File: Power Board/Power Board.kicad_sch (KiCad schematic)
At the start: 126 parts, among them IC1 LTC4151IMS#PBF, J8 Conn_01x02, K1 Relay_DPST-NO, Q10 Q_NMOS_GDS, Q11 Q_NMOS_GDS, Q12 Q_NMOS_GDS, Q13 Q_NMOS_GDS, Q14 Q_NMOS_GDS, Q15 Q_NMOS_GDS, Q16 Q_NMOS_GDS, Q17 Q_NMOS_GDS, Q18 Q_NMOS_GDS, Q19 Q_NMOS_GDS, Q20 Q_NMOS_GDS, Q21 Q_NMOS_GDS, Q22 Q_NMOS_GDS, Q9 Q_NMOS_GDS, Q9 Q_PMOS_GDS, U1 ADR395, U10 LTC4372, U11 ACS770xCB-200U-PFF, U2 LTC4372, U3 LTC4372, U4 LTC4372, U5 LTC4372, U6 LTC4372, U7 LTC4372, U8 ADC128S052CIMT, U9 L7805

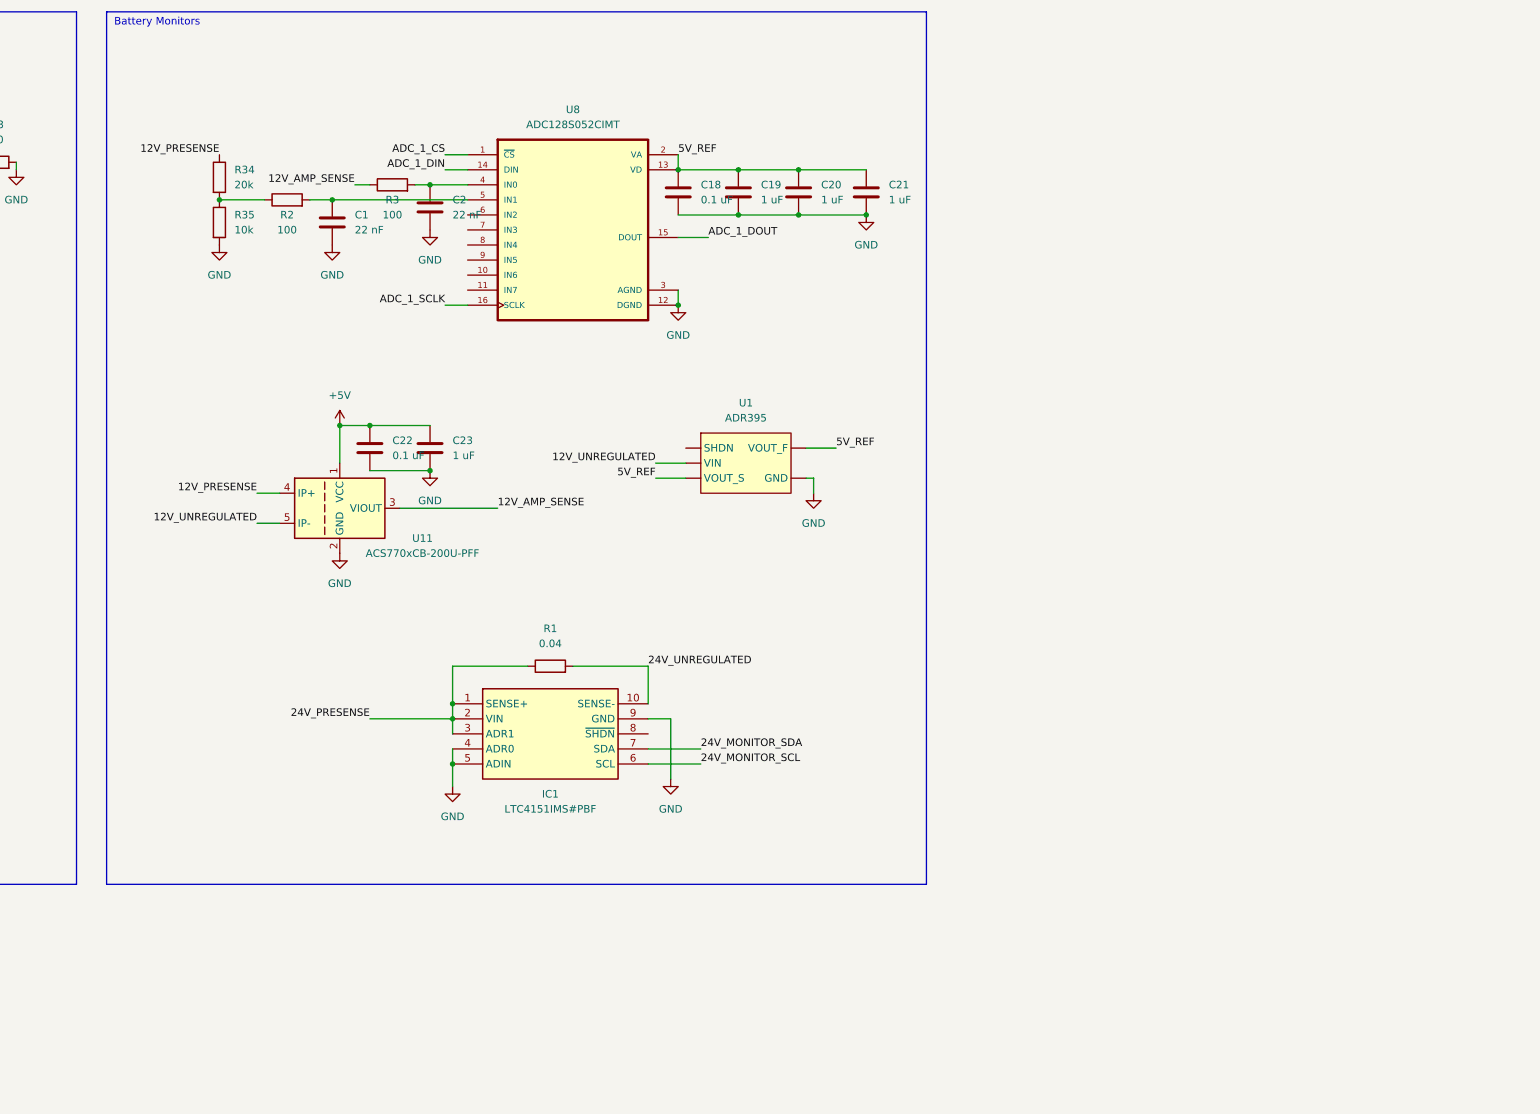
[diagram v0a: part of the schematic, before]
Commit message: working on power board
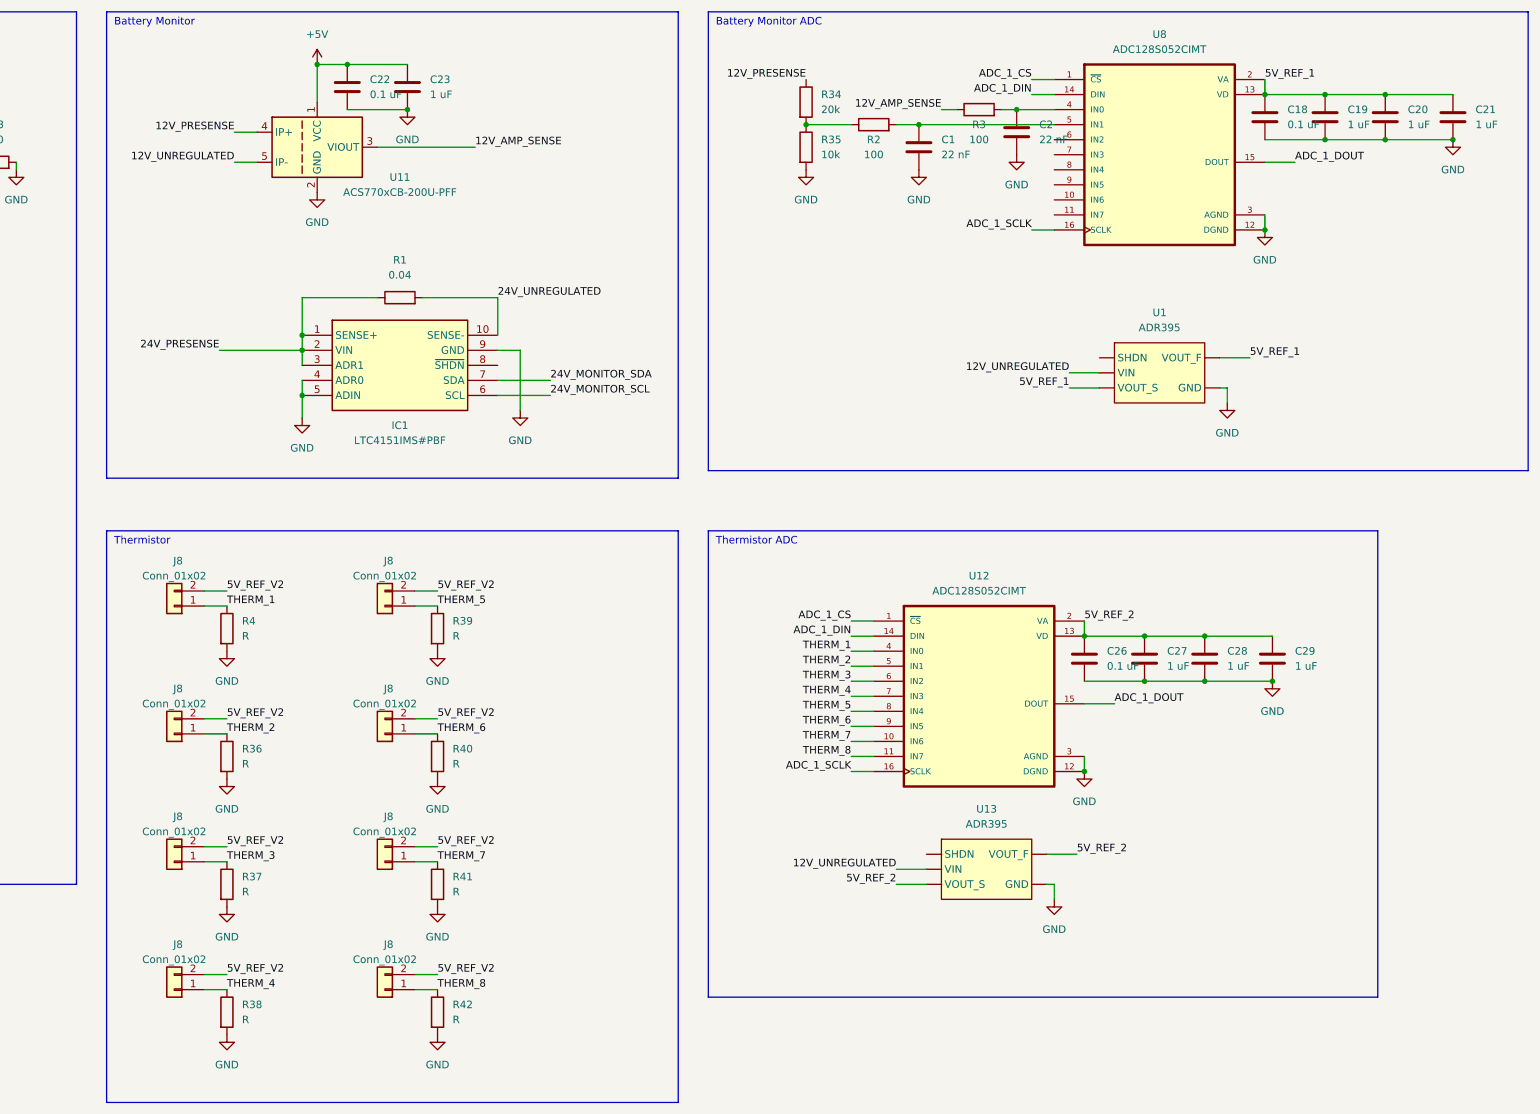
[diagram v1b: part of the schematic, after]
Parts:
- added C26: 0.1 uF, symbol Device:C
- added C27, C28, C29: 1 uF, symbol Device:C
- added J8 (x8): Conn_01x02, SOCMonitor:MOLEX_768290102, symbol Connector_Generic:Conn_01x02
- added R36, R37, R38, R39, R4, R40, R41, R42: R, symbol Device:R
- added U12: ADC128S052CIMT, ADC128S052CIMT:SOP65P640X120-16N, symbol ADC128S052CIMT:ADC128S052CIMT
- added U13: ADR395, Package_TO_SOT_SMD:SOT-23-5, symbol ADR395:ADR395
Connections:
- net 12V_UNREGULATED: now also U13. (VOUT_S)
- net ADC_1_CS: now also U12.1 (~{CS})
- net ADC_1_DIN: now also U12.14 (DIN)
- net ADC_1_DOUT: now also U12.15 (DOUT)
- net ADC_1_SCLK: now also U12.16 (SCLK)
- net GND: now also C26.2, C27.2, C28.2, C29.2, R36.2, R37.2, R38.2, R39.2, R4.2, R40.2, R41.2, R42.2, U12.12 (DGND), U12.3 (AGND), U13. (VOUT_S)
- net 5V_REF renamed 5V_REF_1
- new net 5V_REF_2: C26.1, C27.1, C28.1, C29.1, U12.13 (VD), U12.2 (VA), U13. (VOUT_S)
- new net 5V_REF_V2: J8.2 (Pin_2), J8.2 (Pin_2), J8.2 (Pin_2), J8.2 (Pin_2), J8.2 (Pin_2), J8.2 (Pin_2), J8.2 (Pin_2), J8.2 (Pin_2)
- new net THERM_1: J8.1 (Pin_1), R4.1, U12.4 (IN0)
- new net THERM_2: J8.1 (Pin_1), R36.1, U12.5 (IN1)
- new net THERM_3: J8.1 (Pin_1), R37.1, U12.6 (IN2)
- new net THERM_4: J8.1 (Pin_1), R38.1, U12.7 (IN3)
- new net THERM_5: J8.1 (Pin_1), R39.1, U12.8 (IN4)
- new net THERM_6: J8.1 (Pin_1), R40.1, U12.9 (IN5)
- new net THERM_7: J8.1 (Pin_1), R41.1, U12.10 (IN6)
- new net THERM_8: J8.1 (Pin_1), R42.1, U12.11 (IN7)
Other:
- note added: "Battery Monitor"
- note added: "Battery Monitor ADC"
- note added: "Thermistor"
- note added: "Thermistor ADC"
- note removed: "Battery Monitors"
- moved on the sheet: C1, C18, C19, C2, C20, C21, C22, C23, IC1, R1, R2, R3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
